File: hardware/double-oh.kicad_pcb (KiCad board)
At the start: 2 copper layers, 81.6 x 14 mm, 43 parts, among them J1 USB_B_Micro, J10 Conn_01x01, J11 Conn_01x01, J2 Conn_01x01, J3 Conn_01x01, J4 Conn_01x01, J5 Conn_01x01, J6 Conn_01x01, J7 Conn_01x01, J8 Conn_01x01, J9 Conn_01x01, Q1 Q_PMOS_GSD, Q2 Q_DUAL_NPN_NPN_E1B1C2E2B2C1, U1 AP2127N-3.3, U2 MCP4017-xxxx, U3 MCP73831-2-OT, U4 LMV321, U5 ESP8285, U6 CP2105, Y1 Crystal_GND24

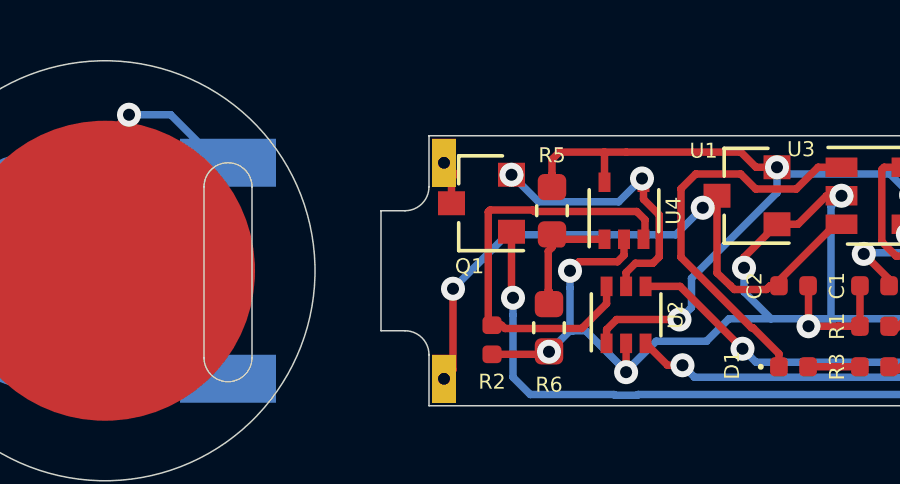
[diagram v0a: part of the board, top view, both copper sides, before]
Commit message: Update main board gerbers
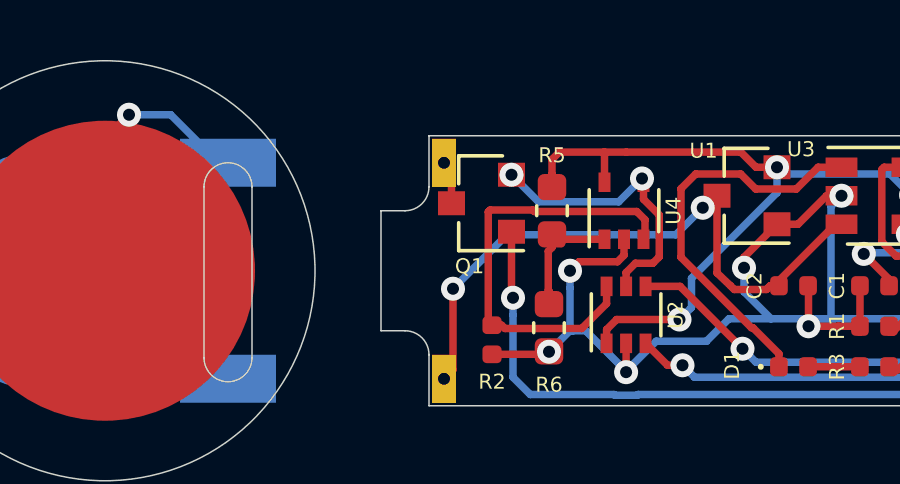
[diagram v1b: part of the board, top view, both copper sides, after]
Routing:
- net to_top_cap: track 2.02 -> 1.45 mm
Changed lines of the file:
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@@
     (thickness 0.6)
     (drawings 58)
-    (tracks 506)
+    (tracks 505)
     (zones 0)
     (modules 43)
@@
   (segment (start 116.362659 103.687339) (end 115.96266 103.28734) (width 0.25) (layer F.Cu) (net 2))
   (segment (start 115.335 105) (end 115.335 104.780819) (width 0.25) (layer F.Cu) (net 2))
+  (segment (start 128.625 106.75) (end 128.625 106.975) (width 0.25) (layer F.Cu) (net 3))
+  (segment (start 128.3 103.65) (end 129.25 103.65) (width 0.25) (layer F.Cu) (net 3))
+  (segment (start 128.224999 103.725001) (end 128.3 103.65) (width 0.25) (layer F.Cu) (net 3))
+  (segment (start 128.224999 106.210001) (end 128.224999 103.725001) (width 0.25) (layer F.Cu) (net 3))
+  (segment (start 128.665 106.650002) (end 128.224999 106.210001) (width 0.25) (layer F.Cu) (net 3))
+  (segment (start 128.665 106.75) (end 128.665 106.650002) (width 0.25) (layer F.Cu) (net 3))
+  (segment (start 129.55 103.35) (end 129.25 103.65) (width 0.25) (layer F.Cu) (net 3))
+  (segment (start 131.6375 103.35) (end 129.55 103.35) (width 0.25) (layer F.Cu) (net 3))
   (segment (start 114.365 107.7) (end 112.635 107.7) (width 0.25) (layer F.Cu) (net 4))
   (segment (start 112.97 101.05) (end 113.75 101.05) (width 0.25) (layer F.Cu) (net 5))
@@
   (segment (start 111.37 105) (end 111.665 105) (width 0.25) (layer F.Cu) (net 7))
   (via (at 132.525 107.85) (size 0.8) (drill 0.4) (layers F.Cu B.Cu) (net 8))
-  (via (at 106.57 107.88) (size 0.8) (drill 0.4) (layers F.Cu B.Cu) (net 8))
   (via (at 104.7 104.5) (size 0.8) (drill 0.4) (layers F.Cu B.Cu) (net 8))
   (via (at 110.5 104.4) (size 0.8) (drill 0.4) (layers F.Cu B.Cu) (net 8))
@@
   (segment (start 140.781484 107.09999) (end 141.10001 107.418516) (width 0.25) (layer F.Cu) (net 8))
   (segment (start 106.5 103.6) (end 106.5 103.98359) (width 0.25) (layer F.Cu) (net 8))
-  (segment (start 106.57 107.85) (end 106.57 107.88) (width 0.25) (layer B.Cu) (net 8))
   (segment (start 110 106.1) (end 109.25 106.85) (width 0.25) (layer B.Cu) (net 8))
   (segment (start 138.55 107.85) (end 139.1 107.3) (width 0.25) (layer B.Cu) (net 8))
@@
   (segment (start 110.5 104.4) (end 110.5 104.05) (width 0.25) (layer F.Cu) (net 8))
   (segment (start 106.5 103.98359) (end 106.28359 104.2) (width 0.25) (layer F.Cu) (net 8))
-  (segment (start 106.57 107.88) (end 106.57 106.92) (width 0.25) (layer F.Cu) (net 8))
   (segment (start 104.8 106.5) (end 104.7 106.4) (width 0.25) (layer B.Cu) (net 8))
   (segment (start 110.5 104.4) (end 110.5 105.2) (width 0.25) (layer B.Cu) (net 8))
@@
   (segment (start 117.215972 104.025972) (end 117.215 104.025) (width 0.25) (layer F.Cu) (net 8))
   (segment (start 124.777644 104.12501) (end 121.92499 104.12501) (width 0.25) (layer B.Cu) (net 8))
-  (segment (start 128.625 106.75) (end 128.625 106.975) (width 0.25) (layer F.Cu) (net 3))
-  (segment (start 128.3 103.65) (end 129.25 103.65) (width 0.25) (layer F.Cu) (net 3))
-  (segment (start 128.224999 103.725001) (end 128.3 103.65) (width 0.25) (layer F.Cu) (net 3))
-  (segment (start 128.224999 106.210001) (end 128.224999 103.725001) (width 0.25) (layer F.Cu) (net 3))
-  (segment (start 128.665 106.650002) (end 128.224999 106.210001) (width 0.25) (layer F.Cu) (net 3))
-  (segment (start 128.665 106.75) (end 128.665 106.650002) (width 0.25) (layer F.Cu) (net 3))
-  (segment (start 129.55 103.35) (end 129.25 103.65) (width 0.25) (layer F.Cu) (net 3))
-  (segment (start 131.6375 103.35) (end 129.55 103.35) (width 0.25) (layer F.Cu) (net 3))
   (segment (start 134.299001 106.874001) (end 134.300001 106.873001) (width 0.25) (layer B.Cu) (net 8))
   (segment (start 122.1 105.25) (end 121.35 106) (width 0.25) (layer F.Cu) (net 8))
@@
   (segment (start 125.252654 103.65) (end 127.05 103.65) (width 0.25) (layer B.Cu) (net 8))
   (segment (start 124.777644 104.12501) (end 125.252654 103.65) (width 0.25) (layer B.Cu) (net 8))
+  (segment (start 106.57 107.85) (end 106.57 107.88) (width 0.25) (layer B.Cu) (net 8))
+  (via (at 106.57 107.88) (size 0.8) (drill 0.4) (layers F.Cu B.Cu) (net 8))
+  (segment (start 106.57 107.88) (end 106.57 106.92) (width 0.25) (layer F.Cu) (net 8))
   (segment (start 128.22 108.625) (end 130.175 108.625) (width 0.25) (layer F.Cu) (net 9))
   (segment (start 130.42498 107.13639) (end 130.52499 107.2364) (width 0.25) (layer F.Cu) (net 9))
@@
   (via (at 102.8 105.4) (size 0.8) (drill 0.4) (layers F.Cu B.Cu) (net 14))
   (via (at 141.125 101.55) (size 0.8) (drill 0.4) (layers F.Cu B.Cu) (net 14))
-  (segment (start 103.375 108.625) (end 102.8 108.05) (width 0.25) (layer B.Cu) (net 14))
-  (segment (start 140.975 108.625) (end 106.968004 108.625) (width 0.25) (layer B.Cu) (net 14))
-  (segment (start 141.125 108.475) (end 140.975 108.625) (width 0.25) (layer B.Cu) (net 14))
-  (segment (start 106.943014 108.64999) (end 106.196986 108.64999) (width 0.25) (layer B.Cu) (net 14))
-  (segment (start 106.196986 108.64999) (end 106.171996 108.625) (width 0.25) (layer B.Cu) (net 14))
-  (segment (start 102.8 108.05) (end 102.8 105.965685) (width 0.25) (layer B.Cu) (net 14))
-  (segment (start 102.8 105.965685) (end 102.8 105.4) (width 0.25) (layer B.Cu) (net 14))
-  (segment (start 141.125 101.55) (end 141.125 108.475) (width 0.25) (layer B.Cu) (net 14))
-  (segment (start 106.171996 108.625) (end 103.375 108.625) (width 0.25) (layer B.Cu) (net 14))
   (segment (start 135.37 100.65) (end 135.665 100.65) (width 0.25) (layer F.Cu) (net 14))
   (segment (start 139.999999 100.424999) (end 140.725001 101.150001) (width 0.25) (layer F.Cu) (net 14))
   (segment (start 135.665 100.65) (end 135.890001 100.424999) (width 0.25) (layer F.Cu) (net 14))
   (segment (start 102.75 103.2) (end 102.75 105.35) (width 0.25) (layer F.Cu) (net 14))
-  (segment (start 106.968004 108.625) (end 106.943014 108.64999) (width 0.25) (layer B.Cu) (net 14))
   (segment (start 140.725001 101.150001) (end 141.125 101.55) (width 0.25) (layer F.Cu) (net 14))
   (segment (start 135.890001 100.424999) (end 139.999999 100.424999) (width 0.25) (layer F.Cu) (net 14))
   (segment (start 102.75 105.35) (end 102.8 105.4) (width 0.25) (layer F.Cu) (net 14))
+  (segment (start 106.943014 108.64999) (end 106.196986 108.64999) (width 0.25) (layer B.Cu) (net 14))
+  (segment (start 106.968004 108.625) (end 106.943014 108.64999) (width 0.25) (layer B.Cu) (net 14))
+  (segment (start 141.125 101.55) (end 141.125 108.475) (width 0.25) (layer B.Cu) (net 14))
+  (segment (start 106.196986 108.64999) (end 106.171996 108.625) (width 0.25) (layer B.Cu) (net 14))
+  (segment (start 140.975 108.625) (end 106.968004 108.625) (width 0.25) (layer B.Cu) (net 14))
+  (segment (start 102.8 105.965685) (end 102.8 105.4) (width 0.25) (layer B.Cu) (net 14))
+  (segment (start 141.125 108.475) (end 140.975 108.625) (width 0.25) (layer B.Cu) (net 14))
+  (segment (start 106.171996 108.625) (end 103.375 108.625) (width 0.25) (layer B.Cu) (net 14))
+  (segment (start 103.375 108.625) (end 102.8 108.05) (width 0.25) (layer B.Cu) (net 14))
+  (segment (start 102.8 108.05) (end 102.8 105.965685) (width 0.25) (layer B.Cu) (net 14))
   (via (at 107.1 101.425) (size 0.8) (drill 0.4) (layers F.Cu B.Cu) (net 15))
   (segment (start 107.15 102.11359) (end 107.675001 102.638591) (width 0.25) (layer F.Cu) (net 15))
@@
   (segment (start 158.8 104.5) (end 154.800001 108.499999) (width 0.25) (layer B.Cu) (net 53))
   (segment (start 153.099999 108.499999) (end 153.014102 108.414101) (width 0.25) (layer B.Cu) (net 53))
-  (segment (start 100.9 101.3) (end 100.5 100.9) (width 0.25) (layer F.Cu) (net 54))
   (segment (start 100.75 101.15) (end 100.5 100.9) (width 0.25) (layer F.Cu) (net 54))
   (segment (start 100.75 102.25) (end 100.75 101.15) (width 0.25) (layer F.Cu) (net 54))
